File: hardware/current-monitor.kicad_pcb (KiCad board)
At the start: 2 copper layers, 50 x 50 mm, 62 parts, among them J1 SENSE, J2 BATTERY, J3 LCD5110, J4 UART, J5 SWD, J6 JTAG, Q1 MUN5314DW1, U1 AP2210K-3.3, U2 MKL03Z8VFK4, U3 MCP6V71U, U4 MCP6031

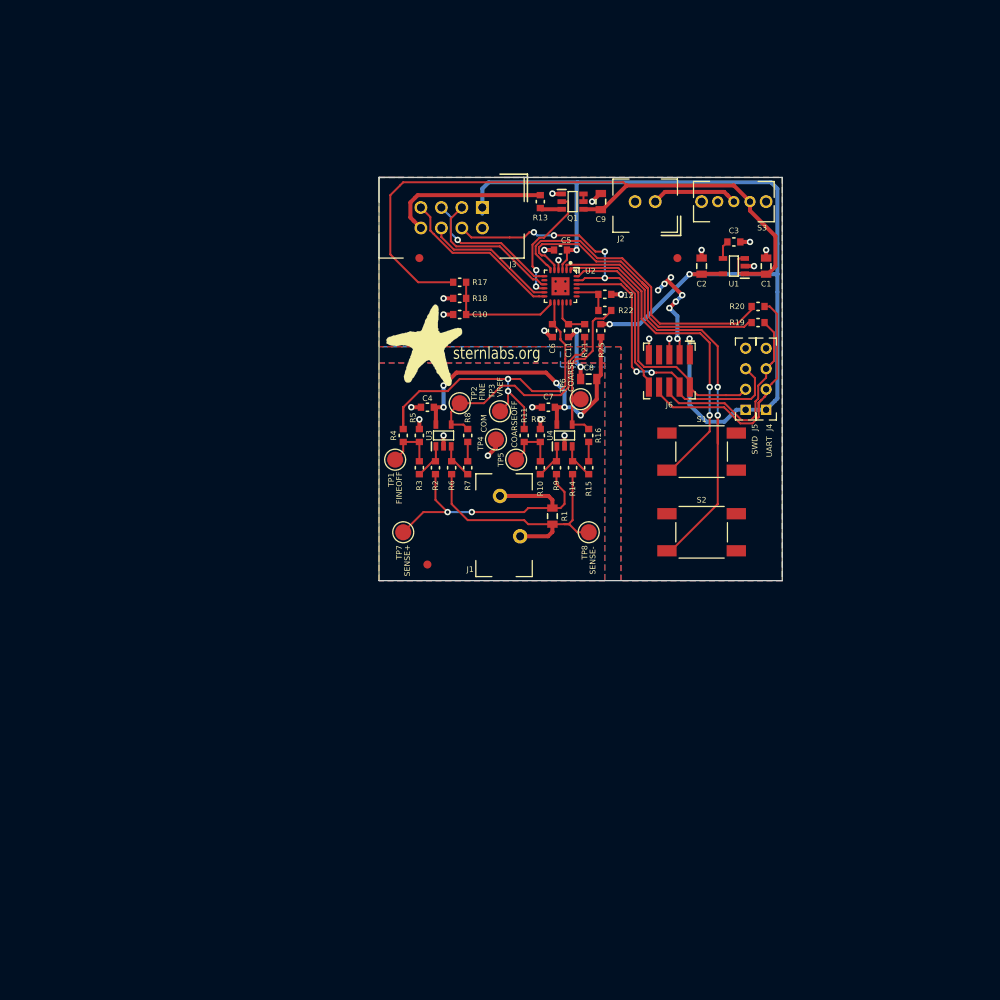
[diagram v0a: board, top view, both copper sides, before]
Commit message: redesign for v1 r1
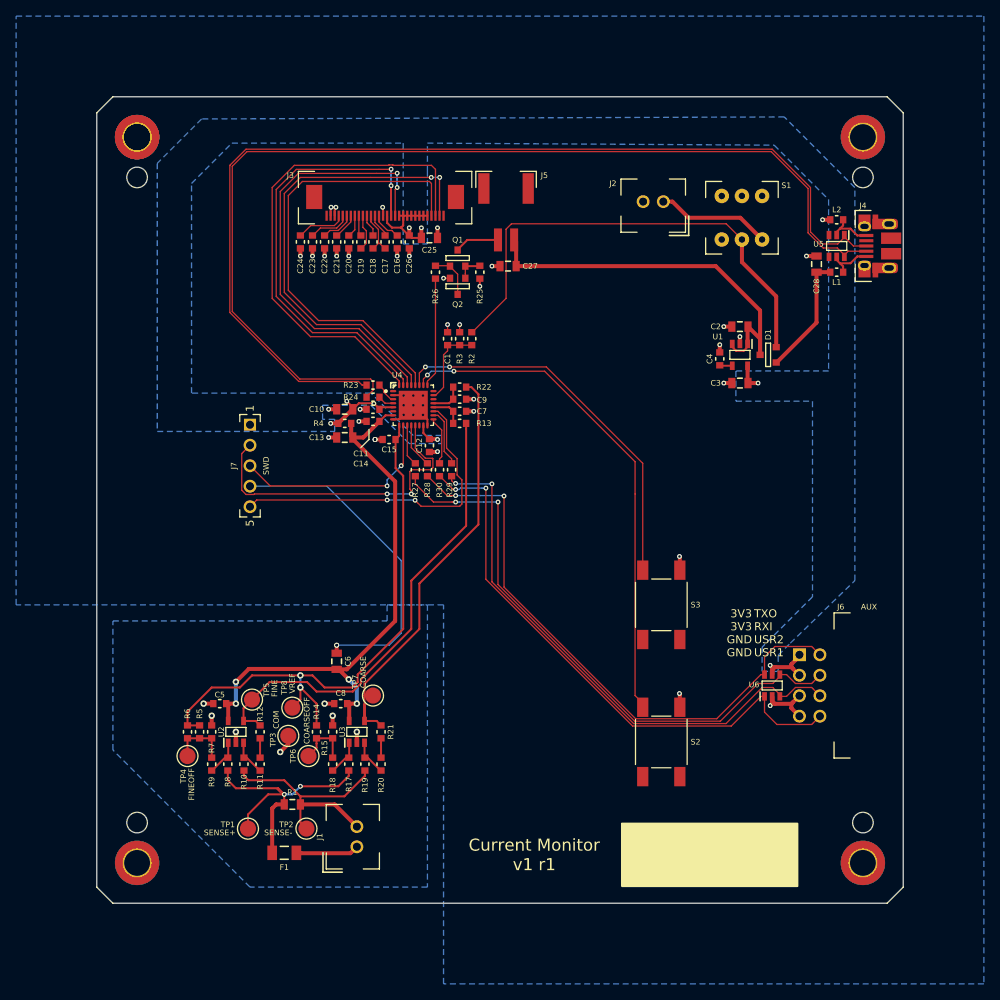
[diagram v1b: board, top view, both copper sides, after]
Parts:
- removed G*** (x2): LOGO, libs:starfish2-10
- removed the R11 at (123.0, 112.0)
- removed the R12 at (125.0, 112.0)
- removed the R4 at (108.0, 112.0)
- removed the REF** at (110.0, 90.0)
- removed the REF** at (142.0, 90.0)
- removed the REF** at (111.0, 128.0)
- removed the S3 at (149.0, 83.0)
- removed the U2 at (127.5, 93.5)
- added C10: 2.2u, libs:SMD-2012, F.Cu at (100.8, 108.8)
- added C11: 0.1u, libs:SMD-1608, F.Cu at (104.2, 108.8)
- added C13: 2.2u, libs:SMD-2012, F.Cu at (100.8, 112.2)
- added C14: 0.1u, libs:SMD-1608, F.Cu at (104.2, 110.2)
- added C16: 1u, libs:SMD-1608, F.Cu at (107.2, 88.0)
- added C17: 1u, libs:SMD-1608, F.Cu at (105.8, 88.0)
- added C18: 1u, libs:SMD-1608, F.Cu at (104.2, 88.0)
- added C19: 1u, libs:SMD-1608, F.Cu at (102.8, 88.0)
- added C20: 1u, libs:SMD-1608, F.Cu at (101.2, 88.0)
- added C21: 1u, libs:SMD-1608, F.Cu at (99.8, 88.0)
- added C22: 1u, libs:SMD-1608, F.Cu at (98.2, 88.0)
- added C23: 1u, libs:SMD-1608, F.Cu at (96.8, 88.0)
- added C24: 1u, libs:SMD-1608, F.Cu at (95.2, 88.0)
- added C25: 2.2u 16V, libs:SMD-2012, F.Cu at (111.2, 87.5)
- added C26: 1u, libs:SMD-1608, F.Cu at (108.8, 88.0)
- added C28: 2.2u 16V, libs:SMD-2012, F.Cu at (159.2, 90.8)
- added D1: BAV70, libs:SOT-23, F.Cu at (153.2, 102.0)
- added F1: 1.1A, libs:SMD-3216, F.Cu at (93.2, 163.8)
- added HOLE-M3: VAL**, libs:HOLE-M3-COND, F.Cu at (75.0, 165.0)
- added HOLE-M3: VAL**, libs:HOLE-M3-COND, F.Cu at (165.0, 165.0)
- added HOLE-M3 (x2): VAL**, libs:HOLE-M3-COND, F.Cu at (75.0, 75.0)
- added HOLE-M3: VAL**, libs:HOLE-M3-COND, F.Cu at (165.0, 75.0)
- added J7: SWD, libs:CONN-5-2.54-1.0-PTH, F.Cu at (89.0, 115.8)
- added L1: 22u, libs:SMD-1608, F.Cu at (161.8, 91.8)
- added L2: 22u, libs:SMD-1608, F.Cu at (161.8, 85.2)
- added Q2: 2N2222, libs:SOT-23-BJT, F.Cu at (114.8, 93.5)
- added R14: 100k, libs:SMD-1608, F.Cu at (97.2, 148.8)
- added R15: 499, libs:SMD-1608, F.Cu at (99.2, 148.8)
- added R23: 33, libs:SMD-1608, F.Cu at (104.2, 105.8)
- added R24: 33, libs:SMD-1608, F.Cu at (104.2, 107.2)
- added R26: 1k, libs:SMD-1608, F.Cu at (112.0, 91.8)
- added R28: 1k, libs:SMD-1608, F.Cu at (111.0, 116.2)
- added R30: 1k, libs:SMD-1608, F.Cu at (112.5, 116.2)
- added R6: 100k, libs:SMD-1608, F.Cu at (81.2, 148.8)
- added R7: 499, libs:SMD-1608, F.Cu at (84.2, 148.8)
- added REF**: stencil8hole, libs:stencil8hole, F.Cu at (75.0, 80.0)
- added REF**: stencil8hole, libs:stencil8hole, F.Cu at (75.0, 160.0)
- added REF**: stencil8hole, libs:stencil8hole, F.Cu at (165.0, 160.0)
- added REF**: stencil8hole, libs:stencil8hole, F.Cu at (165.0, 80.0)
- added S1: POWER, libs:SWITCH-8x8-DPDT, F.Cu at (150.0, 85.0)
- added U4: MKL27ZxxVFM4, libs:MKL27ZxxVFM4, F.Cu at (109.2, 108.2)
- added U5: NUP4114, libs:SOT-23-6, F.Cu at (161.8, 88.5)
- added U6: NUP4114, libs:SOT-23-6, F.Cu at (153.8, 143.0)
- J1: footprint libs:TERM-2-2.5 -> libs:JST-XH-2-PTH-TOP
- J3: value LCD5110 -> ERC12864-1; footprint libs:CONN-2x4-1.0-PTH-SHROUD -> libs:ER-CON30HB-1
- J4: value UART -> USB-MICROB; footprint libs:CONN-4-2.54-0.8-PTH -> libs:USB-MICRO-B-FCI-10103594
- J5: value SWD -> LCD_BL; footprint libs:CONN-4-2.54-0.8-PTH -> libs:ER-CON2.0-2P-SMD
- J6: value JTAG -> AUX; footprint libs:CONN-2x5-1.27-SMT -> libs:CONN-2x4-1.0-PTH-RIGHT-SHROUD
- Q1: value MUN5314DW1 -> 2N2222; footprint libs:SOT-23-6 -> libs:SOT-23-BJT
- R11: renamed from R7; value 1M -> 100k
- R2: renamed from R17; value 1M -> 100k
- R25: renamed from R13; value 1k -> 120
- R27: renamed from R19; value 499 -> 1k
- R29: renamed from R20; value 499 -> 1k
- R5: value 536 -> 100k
- R9: renamed from R3; value 1M -> 100k
- U2: renamed from U3; value MCP6V71U -> MCP6V81U
- U3: renamed from U4; value MCP6031 -> MCP6001U
- moved TP2 50.8 mm to (96.0, 160.8), turned to 0 degrees
- moved R1 48.1 mm to (94.2, 157.8), turned to 90 degrees
- moved C6 46.9 mm to (99.8, 140.0), turned to 180 degrees
- moved R27 46.3 mm to (109.5, 116.2), turned to 0 degrees
- moved R5 45.8 mm to (82.8, 148.8)
- moved C5 44.9 mm to (85.2, 145.2)
- moved C8 44.9 mm to (100.2, 145.2)
- moved R10 44.9 mm to (88.2, 152.8)
- moved R11 44.9 mm to (90.2, 152.8)
- moved R12 44.9 mm to (90.2, 148.8)
- moved R17 44.9 mm to (101.2, 152.8)
- moved R18 44.9 mm to (99.2, 152.8)
- moved R19 44.9 mm to (103.2, 152.8)
- moved R20 44.9 mm to (105.2, 152.8)
- moved R21 44.9 mm to (105.2, 148.8)
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- renumbered C10 to C1, C5 to C12, C6 to C15, C1 to C2, C9 to C27, C2 to C3, C3 to C4, C4 to C5, C8 to C6, C11 to C7, C7 to C8, C12 to C9, R6 to R10, R8 to R12, R21 to R13, R9 to R17, R10 to R18, R14 to R19, R15 to R20, R16 to R21, R18 to R3, R25 to R4, R2 to R8, S1 to S2, S2 to S3, TP7 to TP1, TP8 to TP2, TP4 to TP3, TP1 to TP4, TP2 to TP5, TP5 to TP6, TP6 to TP7, TP3 to TP8
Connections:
- net Net-(C10-Pad1) renamed BAT_SENSE
- C2 pad 1: VBAT -> VIN
- C27 pad 1: VBAT -> VIN
- J1 pad 1: SENSE+ -> Net-(F1-Pad1)
- J3 pad 1: +3V3 -> Net-(J3-Pad1)
- J3 pad 2: COM -> /~LCD_CS
- J3 pad 3: /~LCD_CS -> /~LCD_RES
- J3 pad 4: /~RESET -> /LCD_DATA
- J3 pad 5: /LCD_DATA -> +3V3
- J3 pad 6: /MOSI -> +3V3
- J3 pad 7: /SCLK -> +3V3
- J3 pad 8: Net-(J3-Pad8) -> +3V3
- J4 pad 1: +3V3 -> Net-(J4-Pad1)
- J4 pad 2: /UART_RX -> /USB_DM
- J4 pad 3: /UART_TX -> /USB_DP
- J4 pad 4: COM -> Net-(J4-Pad4)
- J5 pad 1: +3V3 -> VIN
- J5 pad 2: /SWD_DIO -> Net-(J5-Pad2)
- J6 pad 2: /SWD_DIO -> /UART_TX
- J6 pad 3: COM -> +3V3
- J6 pad 4: /SWD_CLK -> /UART_RX
- J6 pad 6: /UART_TX -> /AUX_USR2
- J6 pad 7: Net-(J6-Pad7) -> COM
- J6 pad 8: /UART_RX -> /AUX_USR1
- R25 pad 1: Net-(Q1-Pad3) -> Net-(Q1-PadE)
- R25 pad 2: Net-(J3-Pad8) -> COM
- R27 pad 1: /UART_TX -> Net-(R27-Pad1)
- R27 pad 2: Net-(R19-Pad2) -> /UART_RX
- R29 pad 1: /UART_RX -> Net-(R29-Pad1)
- R29 pad 2: Net-(R20-Pad2) -> /AUX_USR2
- R5 pad 1: COM -> VREF
- U1 pad 1: VBAT -> VIN
- U1 pad 3: VBAT -> VIN
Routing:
- net /USB_DM: track 0.00 -> 129.7 mm
- net /USB_DP: track 0.00 -> 128.1 mm
- net +3V3: track 131.0 -> 38.0 mm, vias 4 -> 8
- net /AUX_USR1: track 0.00 -> 71.3 mm, vias 0 -> 2
- net /AUX_USR2: track 0.00 -> 69.1 mm, vias 0 -> 2
- net /~LCD_RES: track 0.00 -> 61.6 mm
- net /LCD_MOSI: track 0.00 -> 60.8 mm, vias 0 -> 2
- net /LCD_CLK: track 0.00 -> 56.1 mm, vias 0 -> 2
- net VIN: track 0.00 -> 50.7 mm
- net COM: track 51.2 -> 99.0 mm, vias 30 -> 43
- net /UART_TX: track 26.1 -> 73.2 mm, vias 0 -> 2
- net /UART_RX: track 32.3 -> 72.7 mm, vias 0 -> 2
- net /~LCD_CS: track 18.5 -> 58.4 mm, vias 0 -> 2
- net Net-(R19-Pad2): track 38.8 -> 0.00 mm
- net /LCD_DATA: track 17.5 -> 55.8 mm, vias 1 -> 0
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- added copper zone on B.Cu, net +3V3
- removed copper zone on F.Cu, net COM
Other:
- board size 50 x 50 mm -> 100 x 100 mm
- net class Default: trace_width 0.25 -> 0.15; via_dia 0.8 -> 0.6; via_drill 0.4 -> 0.3
- net class power: via_dia 0.8 -> 0.6; via_drill 0.4 -> 0.3
- rule trace_min: 0.2 -> 0.15
- rule via_min_size: 0.4 -> 0.6
- board text added: "3V3 3V3 GND GND"
- board text added: "Current Monitor v1 r1"
- board text added: "TXO RXI USR2 USR1"
- board text removed: "Current Monitor"
- board text removed: "sternlabs.org"
- board text removed: "v1.0 r0"
